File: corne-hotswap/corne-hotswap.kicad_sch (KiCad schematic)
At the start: 61 parts, among them J1 Battery, J2 nice!view, SW1 SW_Push, SW10 SW_Push, SW11 SW_Push, SW12 SW_Push, SW13 SW_Push, SW14 SW_Push, SW15 SW_Push, SW16 SW_Push, SW17 SW_Push, SW18 SW_Push, SW19 SW_Push, SW2 SW_Push, SW20 SW_Push, SW21 SW_Push, SW3 SW_Push, SW4 SW_Push, SW5 SW_Push, SW6 SW_Push, SW7 SW_Push, SW8 SW_Push, SW9 SW_Push, U1 nice!nano

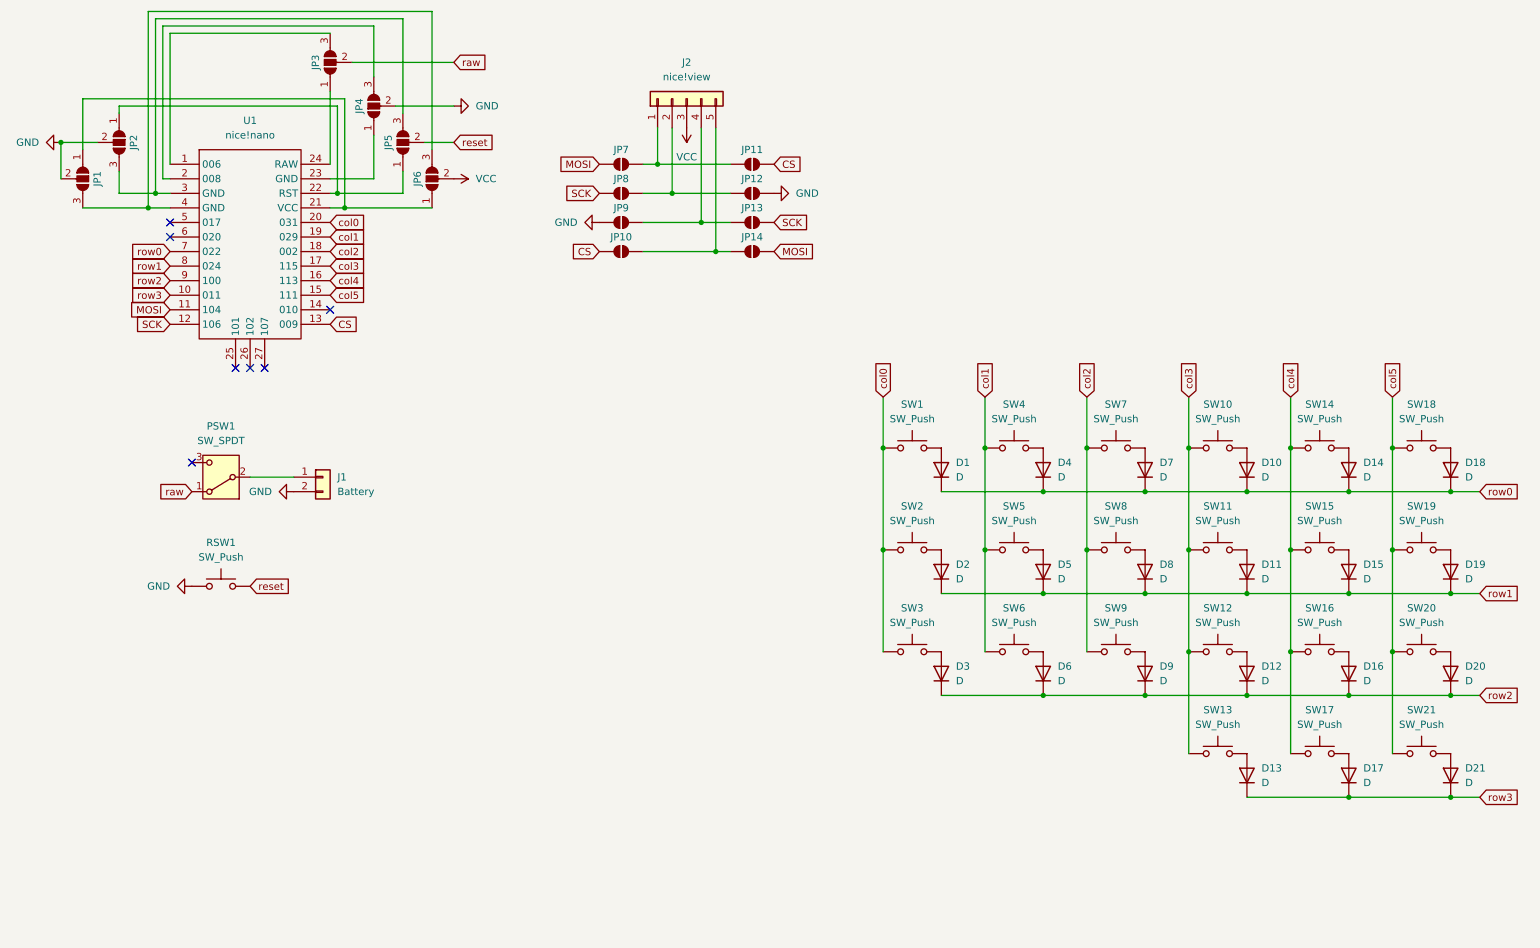
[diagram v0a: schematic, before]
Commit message: Update corne-hotswap.kicad_sch
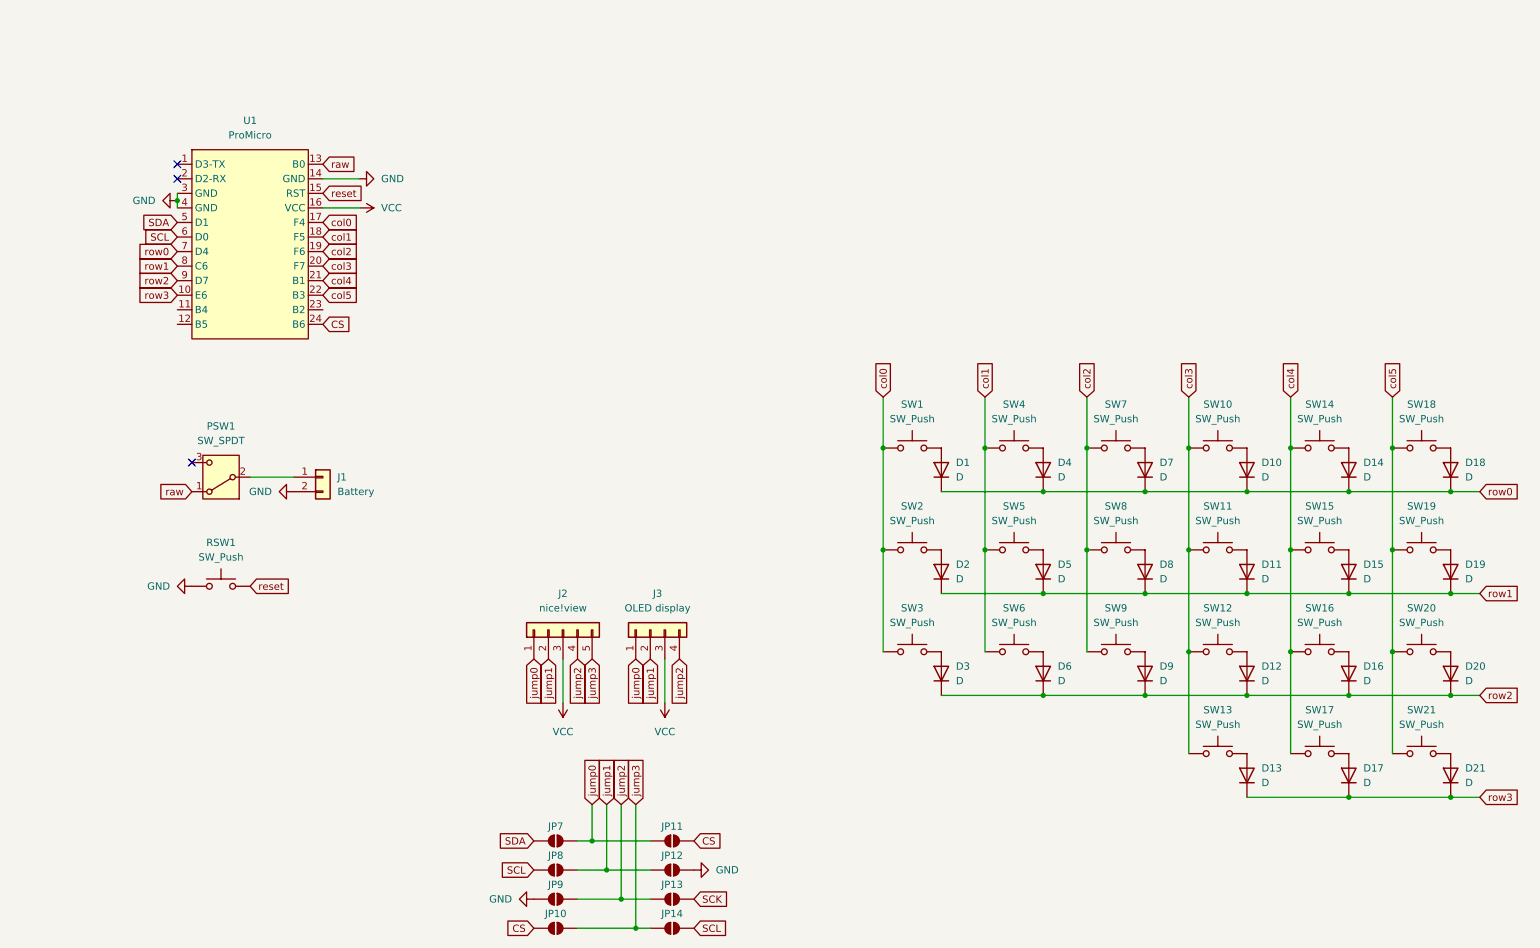
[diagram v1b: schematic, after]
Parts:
- removed JP1, JP2, JP3, JP4, JP5, JP6: SolderJumper_3_Open, symbol Jumper:SolderJumper_3_Open
- removed U1: nice!nano, symbol Corne:NiceNano
- added J3: OLED display, symbol Connector_Generic:Conn_01x04
- added U1: ProMicro, PCM_marbastlib-xp-promicroish:ProMicro_USBup, symbol PCM_marbastlib-promicroish:Arduino_ProMicro
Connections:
- net CS: now also U1.24 (B6)
- net GND: now also U1.14 (GND), U1.3 (GND), U1.4 (GND)
- net SCK: no longer JP8.2 (B)
- net VCC: now also J3.3 (Pin_3), U1.16 (VCC)
- net col0: now also U1.17 (F4)
- net col1: now also U1.18 (F5)
- net col2: now also U1.19 (F6)
- net col3: now also U1.20 (F7)
- net col4: now also U1.21 (B1)
- net col5: now also U1.22 (B3)
- net raw: now also U1.13 (B0)
- net reset: now also U1.15 (RST)
- net row0: now also U1.7 (D4)
- net row1: now also U1.8 (C6)
- net row2: now also U1.9 (D7)
- net row3: now also U1.10 (E6)
- net jump0: now reaches J2.1 (Pin_1), JP11.1 (A), JP7.1 (A)
- net jump0: now also J3.1 (Pin_1)
- net jump2: now reaches J2.4 (Pin_4), JP13.1 (A), JP9.1 (A)
- net jump2: now also J3.4 (Pin_4)
- net jump1: now reaches J2.2 (Pin_2), JP12.1 (A), JP8.1 (A)
- net jump1: now also J3.2 (Pin_2)
- net jump3: now reaches J2.5 (Pin_5), JP10.1 (A), JP14.1 (A)
- net MOSI renamed SCL
- net SCL: now also JP8.2 (B), U1.6 (D0); no longer JP7.2 (B)
- new net SDA: JP7.2 (B), U1.5 (D1)
- no-connect marks 7 -> 3
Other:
- moved on the sheet: JP10, JP11, JP12, JP13, JP14, JP7, JP8, JP9
